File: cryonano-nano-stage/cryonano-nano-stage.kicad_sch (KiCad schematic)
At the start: 7 parts, among them J1 Conn_01x03_Pin

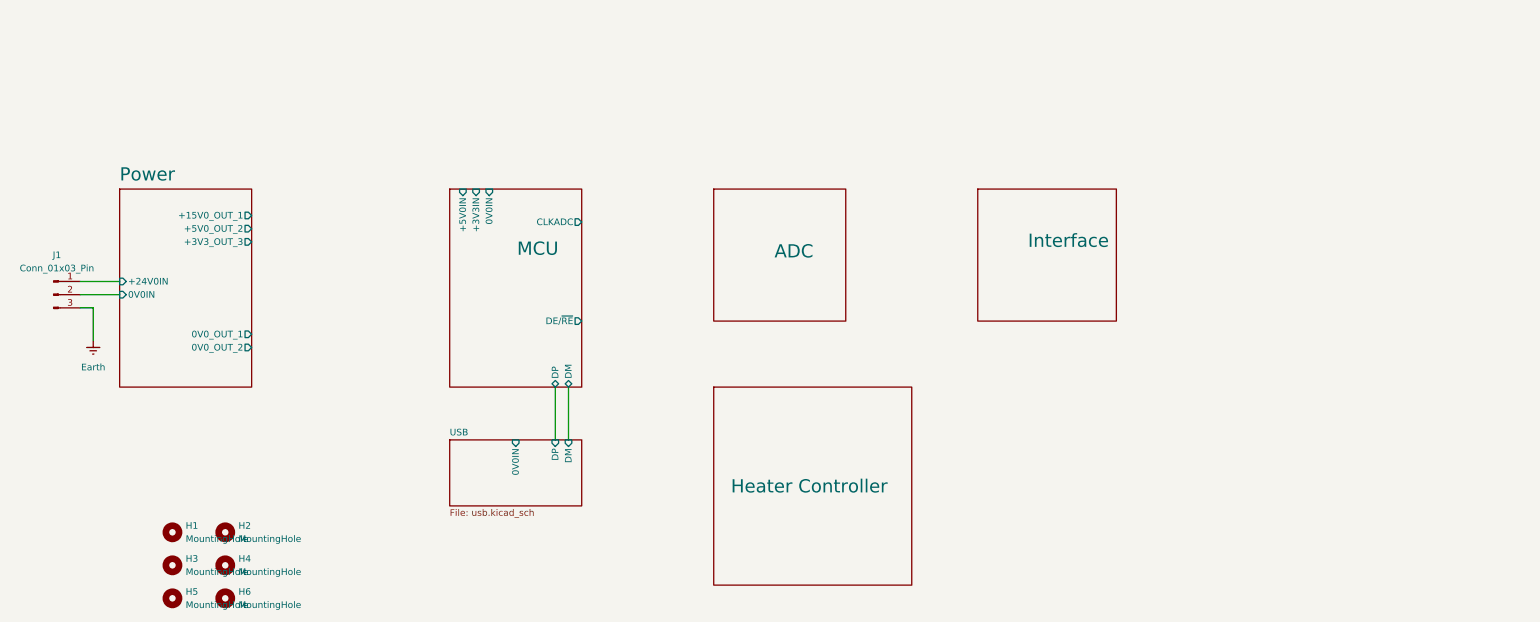
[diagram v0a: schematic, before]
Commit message: sch improved
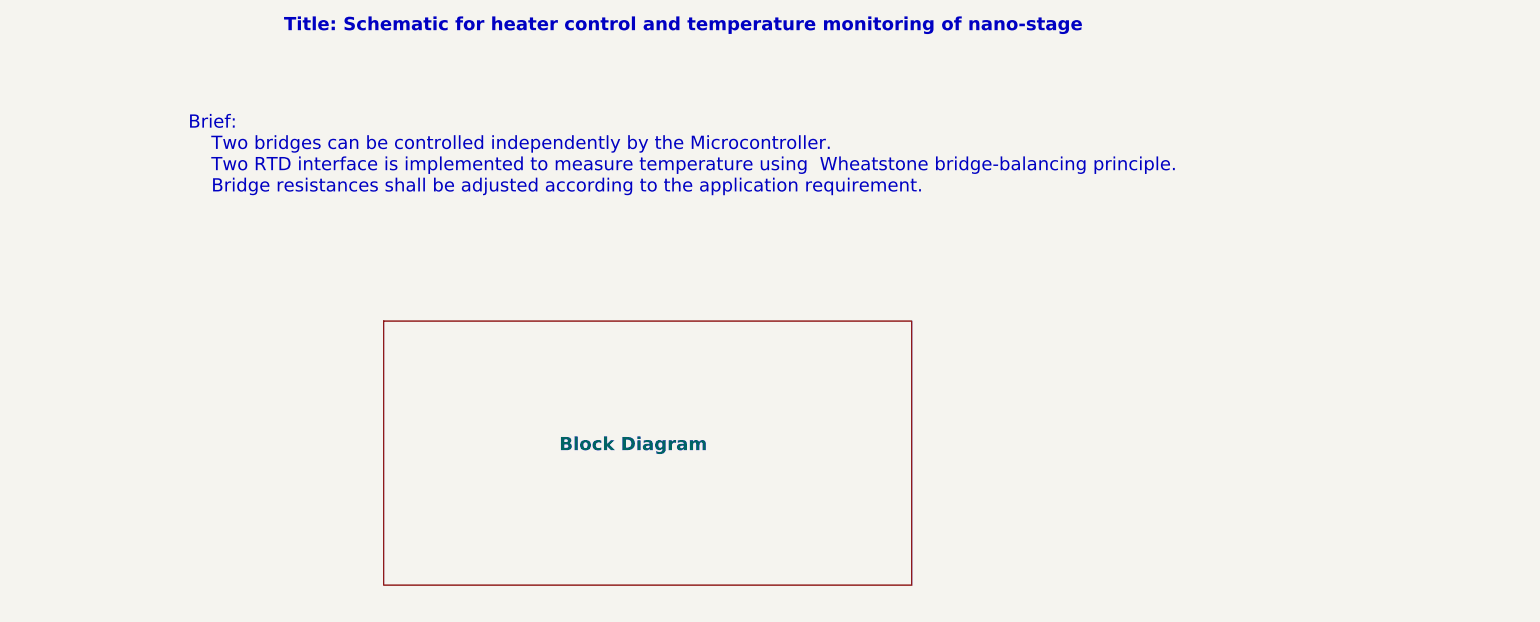
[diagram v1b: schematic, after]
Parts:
- removed H1, H2, H3, H4, H5, H6: MountingHole, footprints:MountingHole_3.7mm_Pad_Small, symbol Mechanical:MountingHole
- removed J1: Conn_01x03_Pin, symbol Connector:Conn_01x03_Pin
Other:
- removed sheet ADC
- removed sheet Heater Controller
- removed sheet Interface
- removed sheet MCU
- removed sheet Power
- removed sheet USB
- added sheet Block Diagram (block-diagram.kicad_sch)
- note added: "Brief: Two bridges can be controlled independently by the Microcontroller. Two RTD interface is implemented to measure temperature using Wheatstone bridge-balancing principle. Bridge resistances shall be adjusted according to the application requirement."
- note added: "Title: Schematic for heater control and temperature monitoring of nano-stage"
